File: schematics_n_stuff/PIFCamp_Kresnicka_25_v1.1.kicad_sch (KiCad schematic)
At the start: 11 parts, among them J1 Conn_01x01_Pin, U1 ATtiny85-20P, U2 TSOP382xx

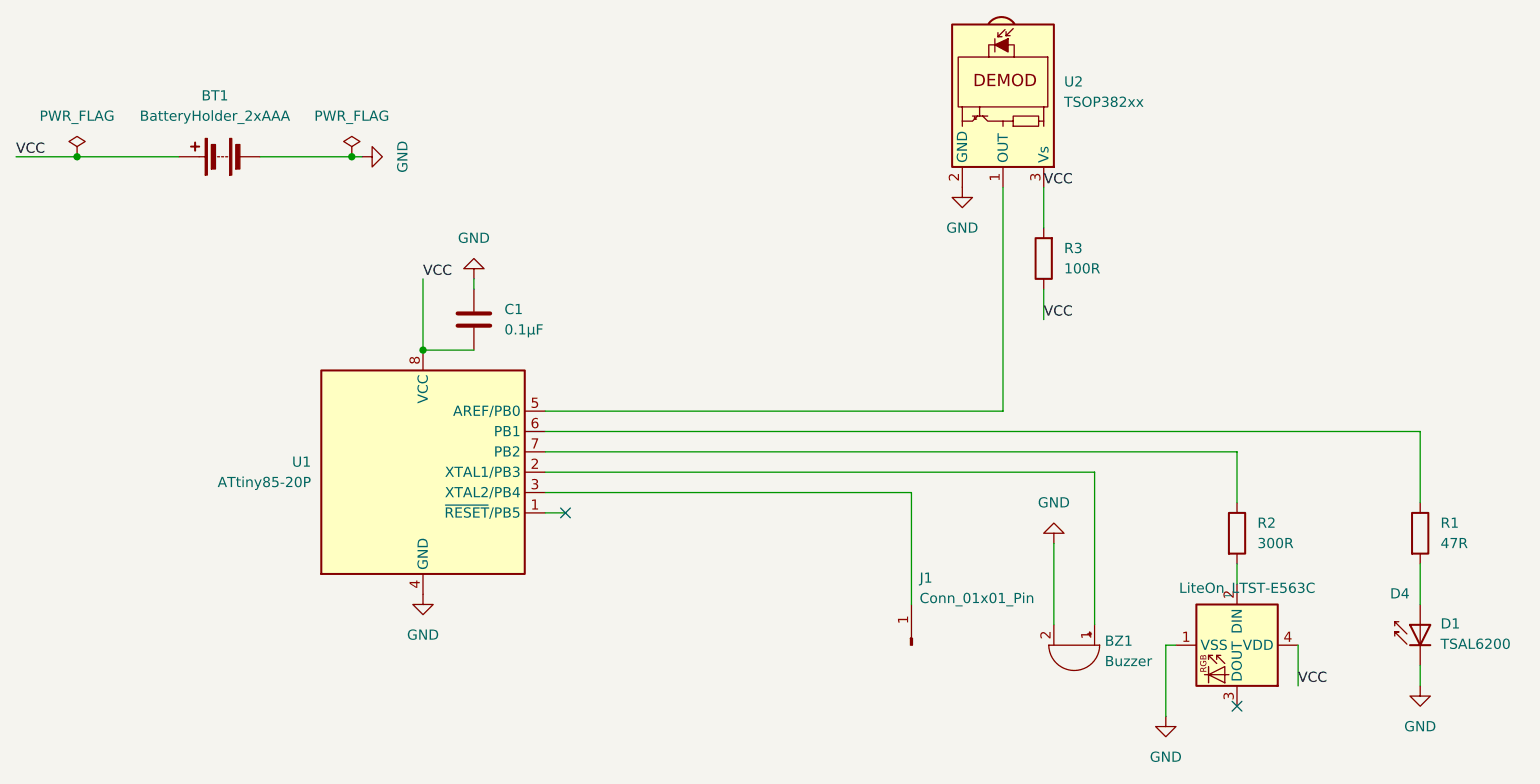
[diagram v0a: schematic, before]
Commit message: panelized
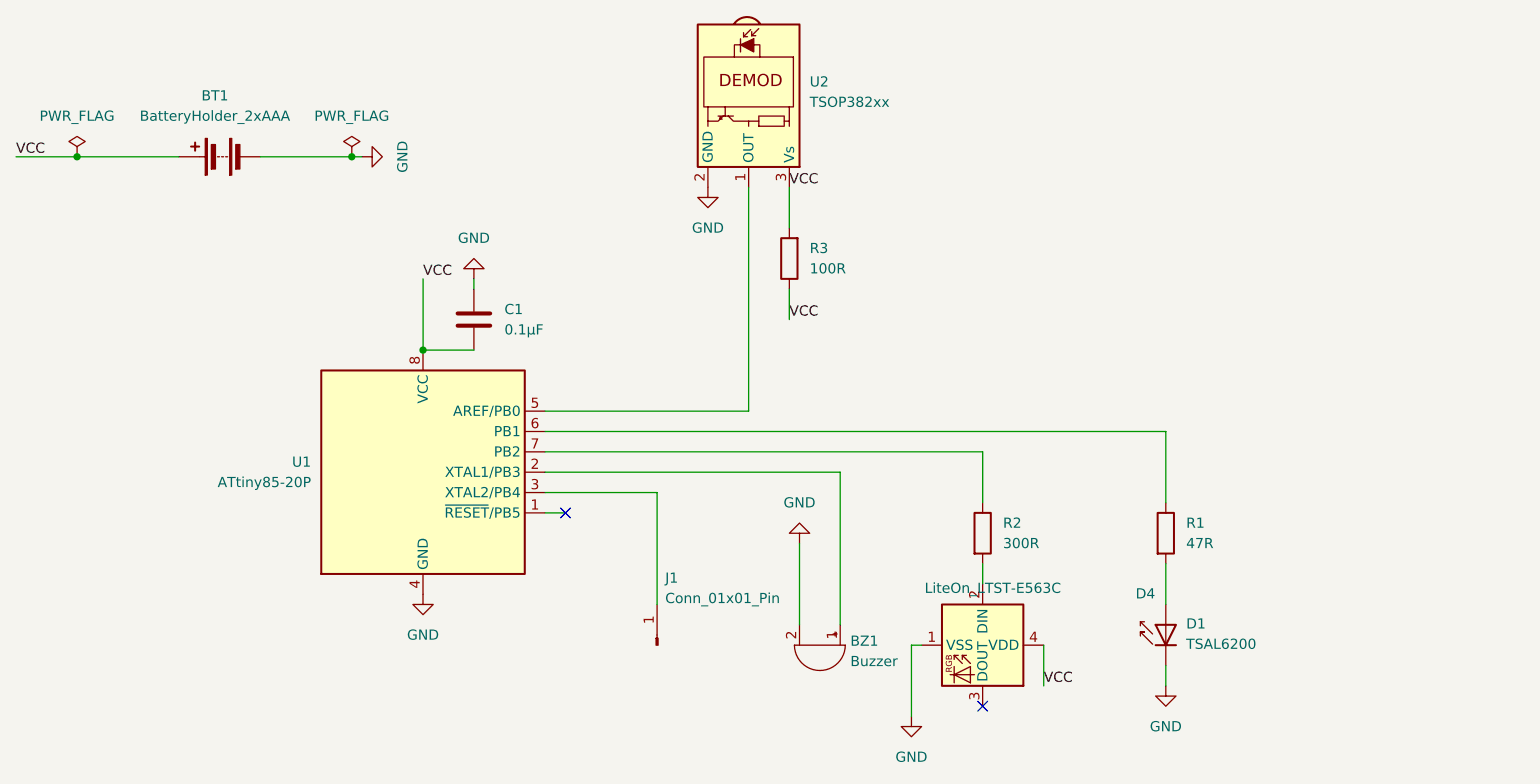
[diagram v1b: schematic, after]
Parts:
- BZ1: footprint Buzzer_Beeper:Buzzer_12x9.5RM7.6 -> Buzzer_Beeper:Buzzer_TDK_PS1240P02BT_D12.2mm_H6.5mm
- U1: footprint Package_DIP:DIP-8_W7.62mm_Socket -> Package_DIP:DIP-8_W7.62mm_LongPads
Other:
- moved on the sheet: BZ1, D1, D4, J1, R1, R2, R3, U2
